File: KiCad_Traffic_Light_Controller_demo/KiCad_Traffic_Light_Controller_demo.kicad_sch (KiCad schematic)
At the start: 40 parts, among them J1 Conn_02x08_Odd_Even, J2 Conn_02x08_Odd_Even, U1 SM420561N, U2 SM420561N

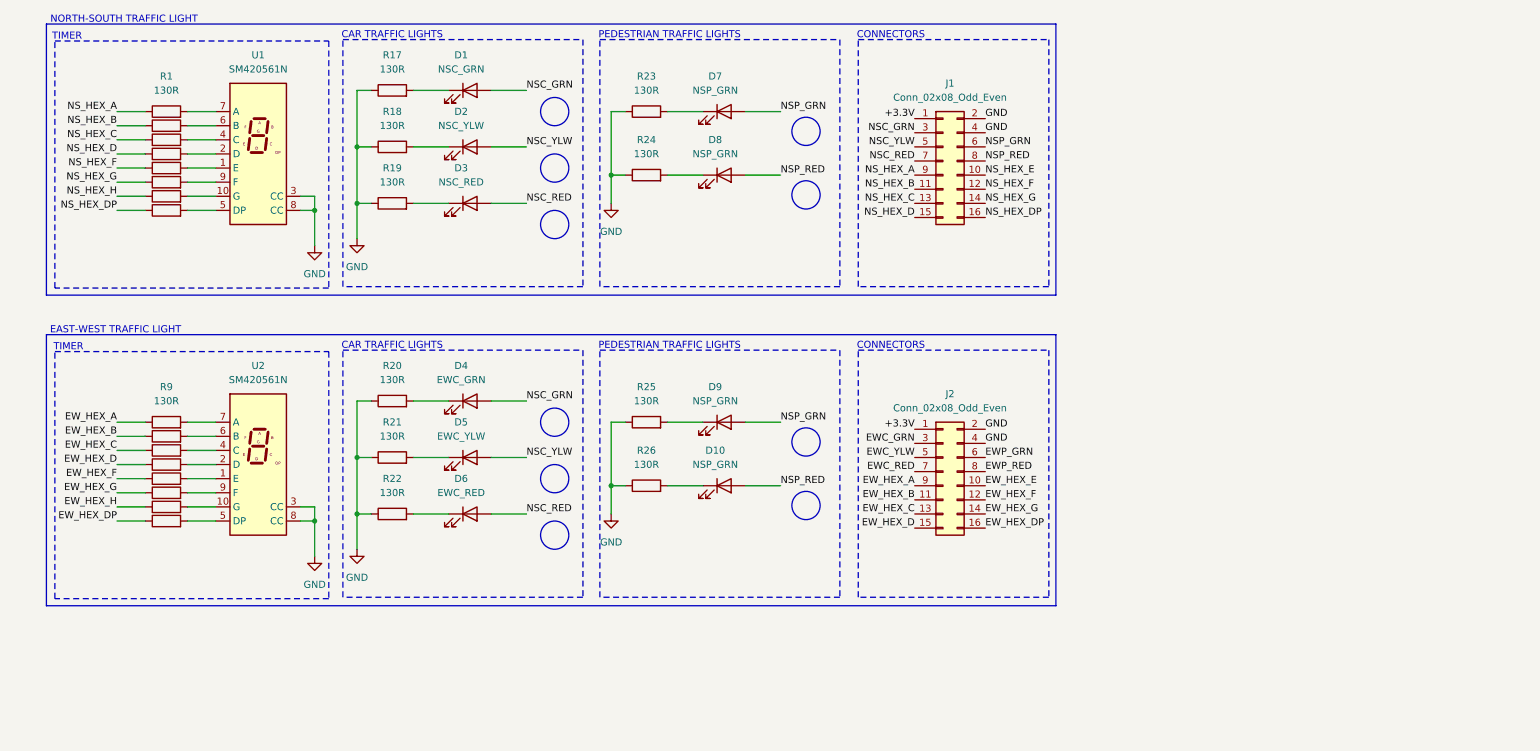
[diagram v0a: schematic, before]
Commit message: Updated KiCad Files
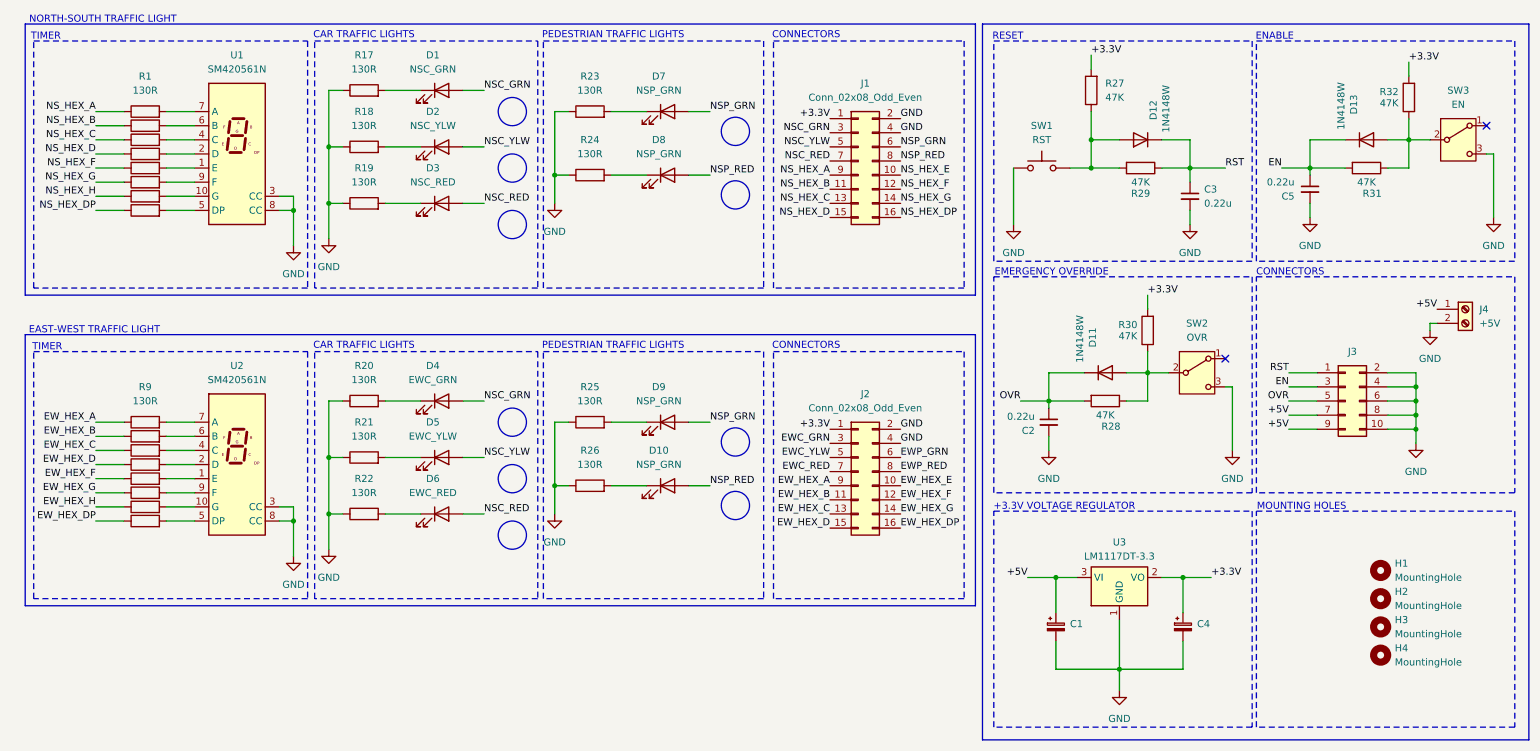
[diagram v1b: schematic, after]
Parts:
- added C1, C4: C_Polarized_Small, symbol Device:C_Polarized_Small
- added C2, C3, C5: 0.22u, symbol Device:C_Small
- added D11, D12, D13: 1N4148W, Diode_SMD:D_SOD-123, symbol Diode:1N4148W
- added H1, H2, H3, H4: MountingHole, symbol Mechanical:MountingHole
- added J3: Conn_02x05_Odd_Even, symbol Connector_Generic:Conn_02x05_Odd_Even
- added J4: +5V, symbol Connector:Screw_Terminal_01x02
- added R27, R28, R29, R30, R31, R32: 47K, symbol Device:R
- added SW1: RST, symbol Switch:SW_Push
- added SW2: OVR, symbol Switch:SW_SPDT
- added SW3: EN, symbol Switch:SW_SPDT
- added U3: LM1117DT-3.3, Package_TO_SOT_SMD:TO-252-3_TabPin2, symbol Regulator_Linear:LM1117DT-3.3
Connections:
- net +3.3V: now also C4.1, R27.2, R30.2, R32.2, U3.2 (VO)
- net GND: now also C1.2, C2.2, C3.2, C4.2, C5.2, J3.10 (Pin_10), J3.2 (Pin_2), J3.4 (Pin_4), J3.6 (Pin_6), J3.8 (Pin_8), J4.2 (Pin_2), SW1.1, SW2.3 (C), SW3.3 (C), U3.1 (GND)
- new net: D13.2 (A), R31.1, R32.1, SW3.2 (B)
- new net: D11.2 (A), R28.1, R30.1, SW2.2 (B)
- new net: D12.2 (A), R27.1, R29.2, SW1.2
- new net +5V: C1.1, J3.7 (Pin_7), J3.9 (Pin_9), J4.1 (Pin_1), U3.3 (VI)
- new net EN: C5.1, D13.1 (K), J3.3 (Pin_3), R31.2
- new net OVR: C2.1, D11.1 (K), J3.5 (Pin_5), R28.2
- new net RST: C3.1, D12.1 (K), J3.1 (Pin_1), R29.1
- no-connect marks 0 -> 2
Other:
- note added: "+3.3V VOLTAGE REGULATOR"
- note added: "EMERGENCY OVERRIDE"
- note added: "ENABLE"
- note added: "MOUNTING HOLES"
- note added: "RESET"
- moved on the sheet: D1, D10, D2, D3, D4, D5, D6, D7, D8, D9, J1, J2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
